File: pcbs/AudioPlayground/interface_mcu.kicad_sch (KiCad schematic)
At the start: 20 parts, among them J4 TC2030, U2 R7FA4M2AB3CNE, Y2 12mHz

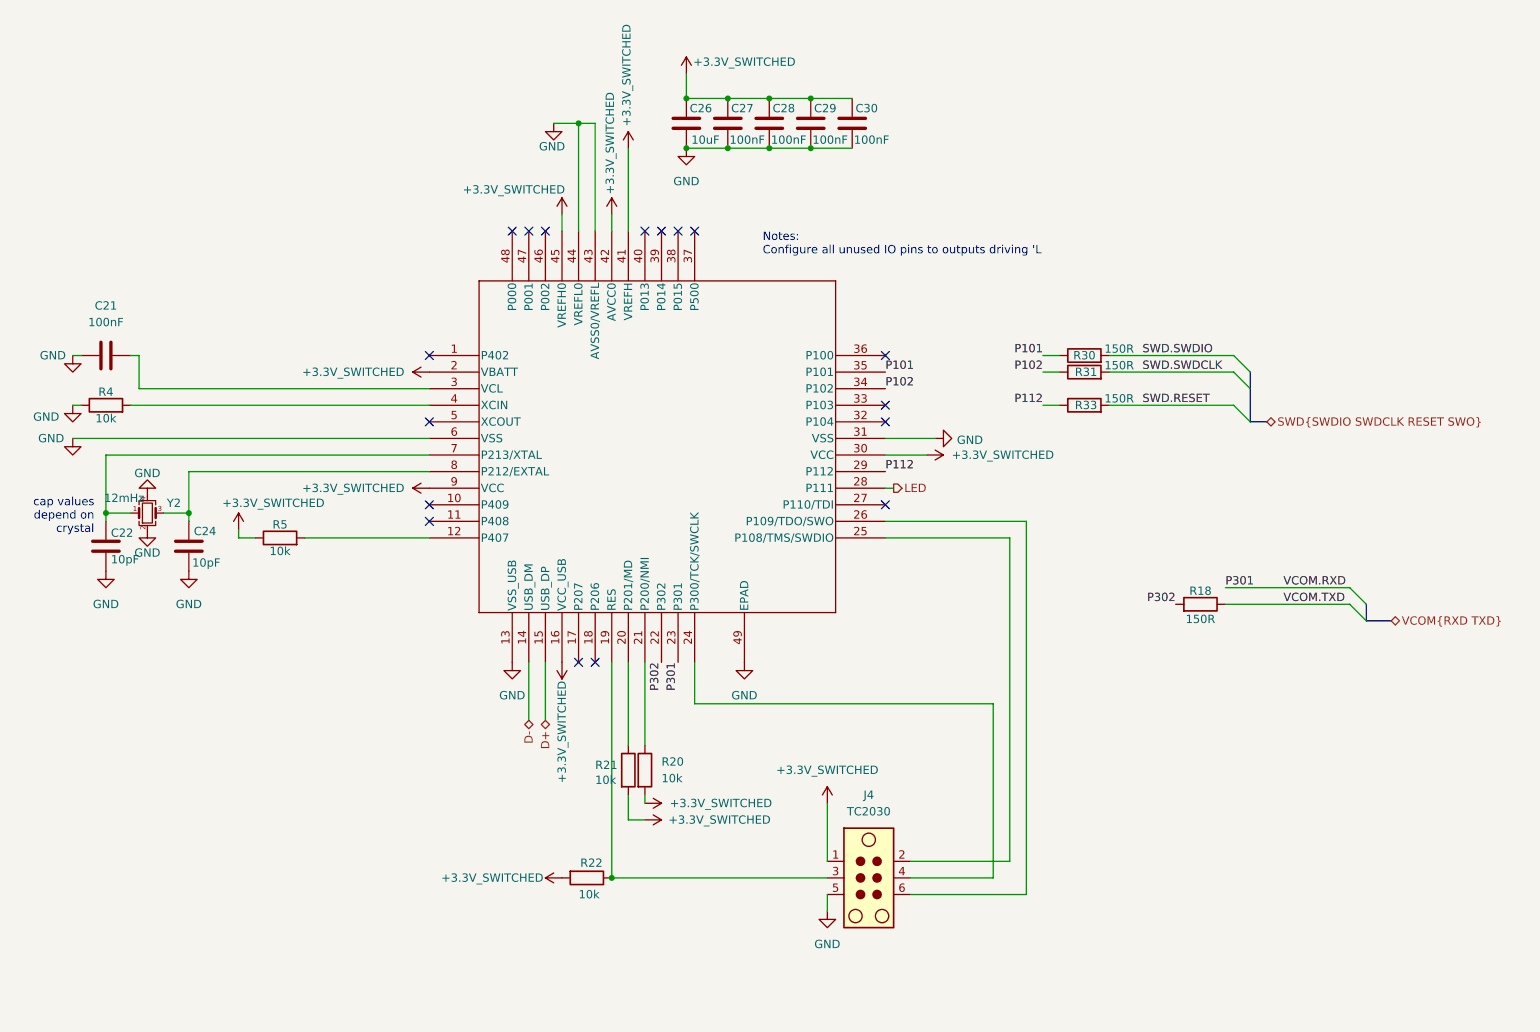
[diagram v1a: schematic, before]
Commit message: Improve Optic
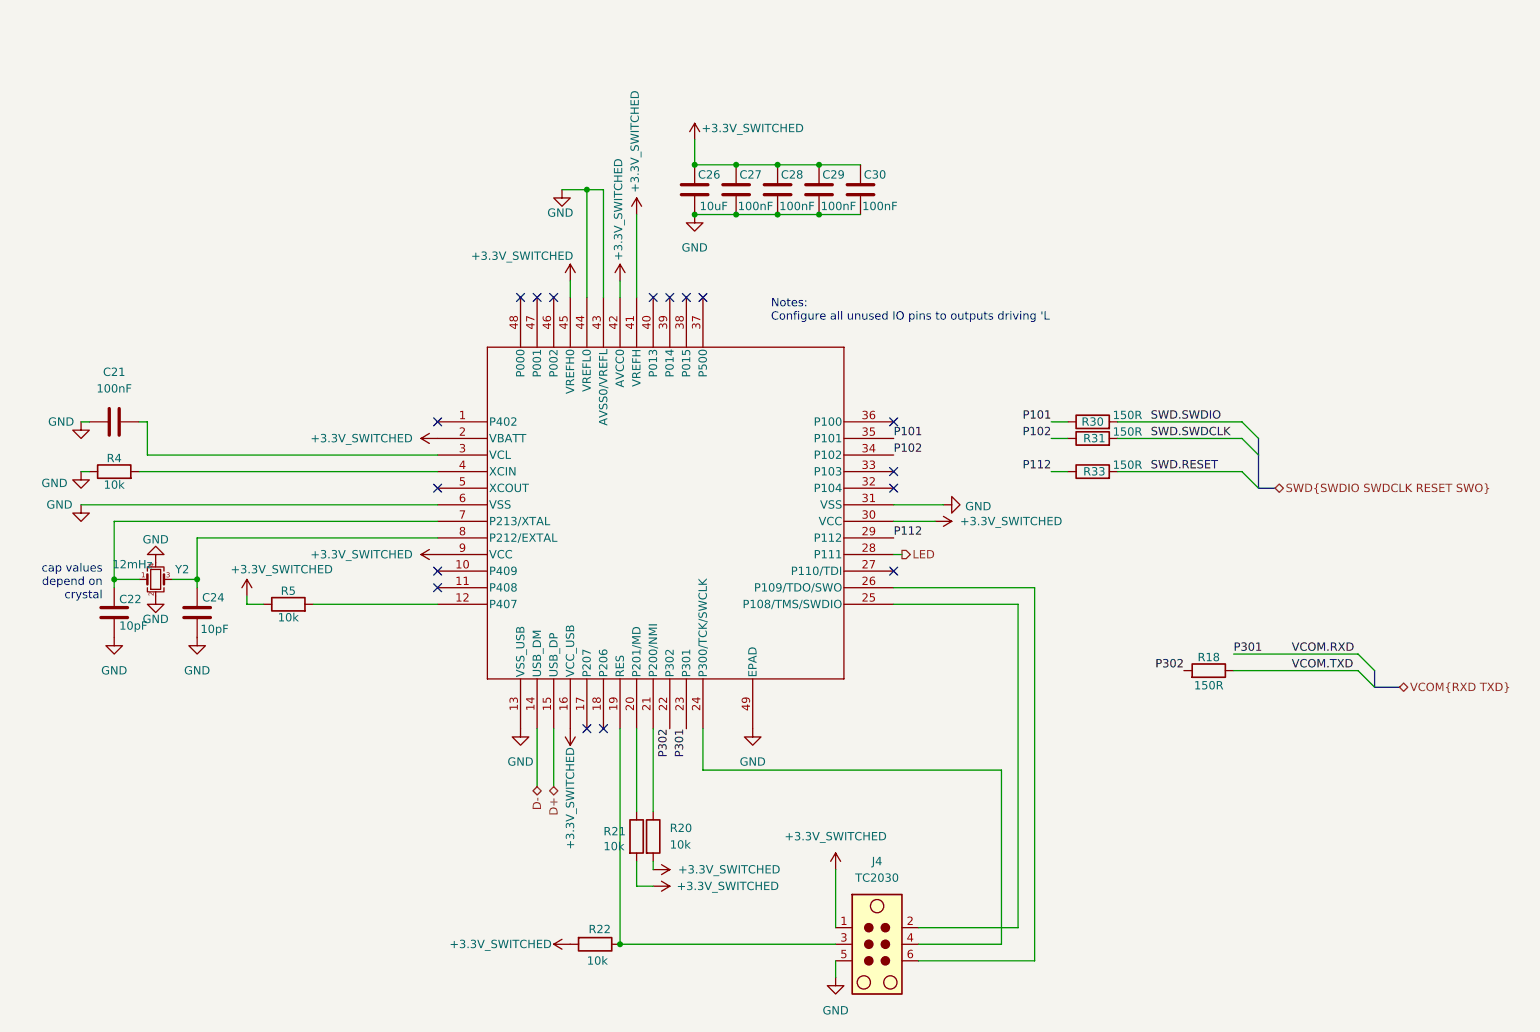
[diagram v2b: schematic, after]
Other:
- title: (none) -> LE Audio Playground
- moved on the sheet: C21, C22, C24, C26, C27, C28, C29, C30, J4, R18, R20, R21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
